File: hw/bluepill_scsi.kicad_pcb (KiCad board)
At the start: 2 copper layers, 43.8 x 73.7 mm, 14 parts, among them J1 Micro_SD_Card, J2 Conn_02x25_Odd_Even, J3 Programming Pins, J4 Berg Power Connector, U1 BluePill_STM32F103C

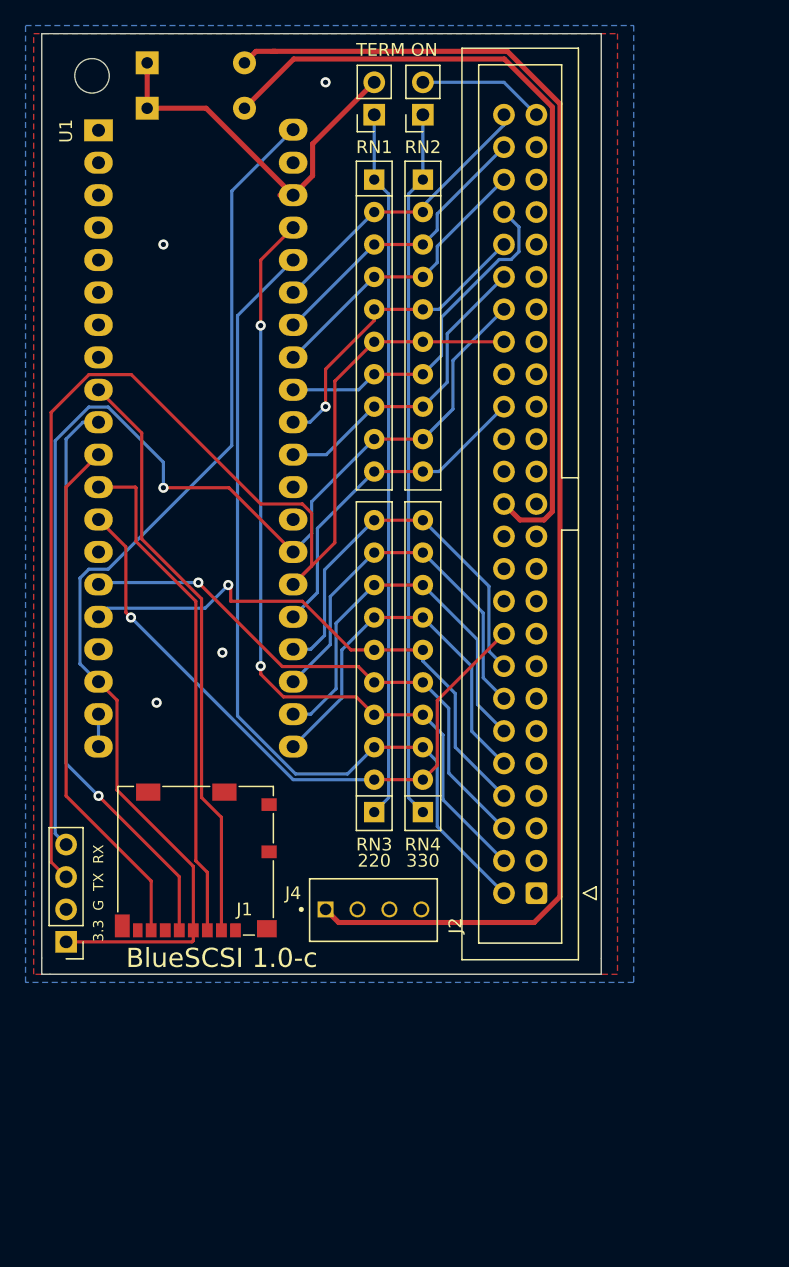
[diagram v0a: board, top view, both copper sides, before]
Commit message: Initial 1.1-a
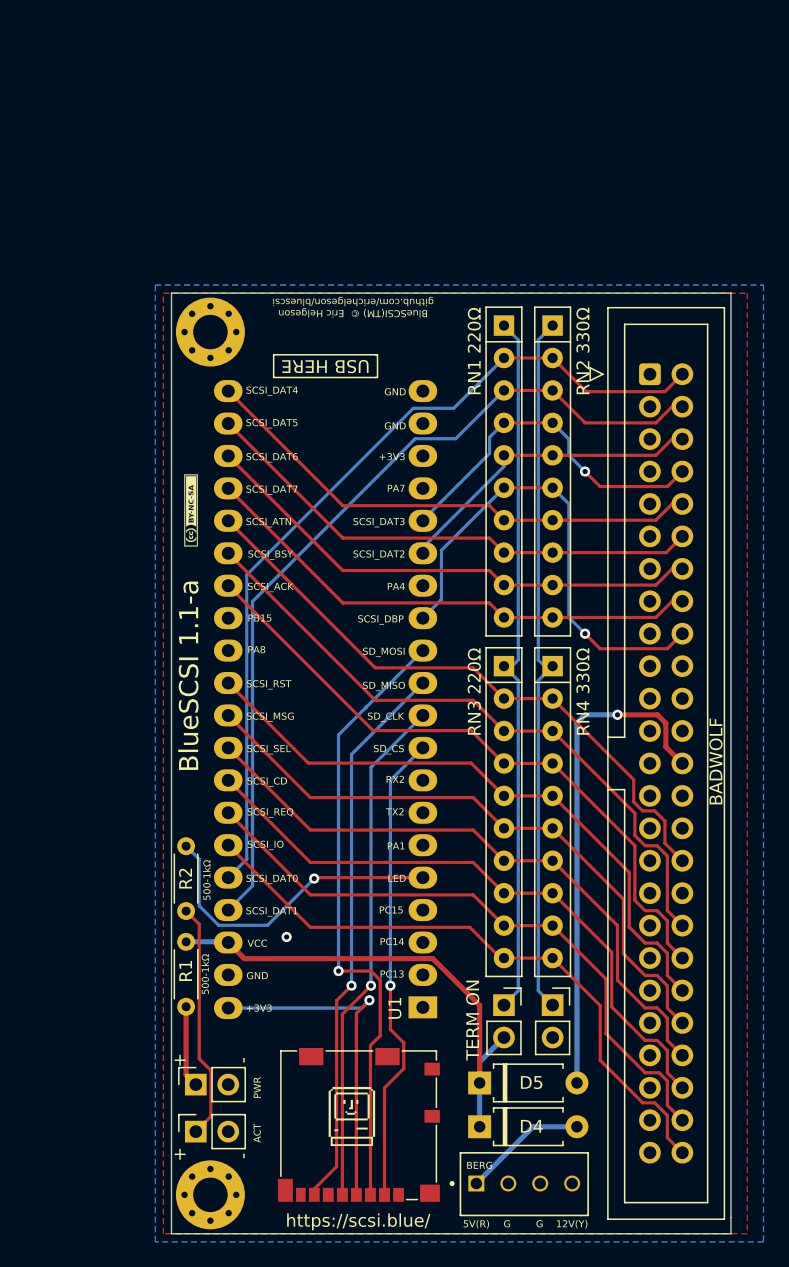
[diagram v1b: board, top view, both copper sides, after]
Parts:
- added G***: LOGO, BlueSCSILogo:dogcow, B.Cu at (95.3, 160.4)
- added G***: LOGO, BlueSCSILogo:mac_happy_small, F.Cu at (95.4, 160.3)
- added G***: LOGO, BlueSCSILogo:cc_by_nc_sa_front_silk_screen, B.Cu at (103.9, 149.4)
- added G***: LOGO, BlueSCSILogo:cc_by_nc_sa_small_front_silk_screen, F.Cu at (82.8, 112.9)
- added G***: LOGO, BlueSCSILogo:BlueSCSILogoFP, B.Cu at (93.2, 126.2)
- added H2: MountingHole_Pad, MountingHole:MountingHole_2.7mm_M2.5_Pad_Via, F.Cu at (84.3, 166.5)
- added J5: Micro_SD_Card, Connector_Card:microSD_HC_Molex_104031-0811, F.Cu at (96.0, 161.0)
- added R1: R_US, Resistor_THT:R_Axial_DIN0204_L3.6mm_D1.6mm_P5.08mm_Horizontal, F.Cu at (82.4, 151.8)
- added R2: R_US, Resistor_THT:R_Axial_DIN0204_L3.6mm_D1.6mm_P5.08mm_Horizontal, F.Cu at (82.4, 144.3)
- D4, D5: moved to F.Cu
- H1: footprint MountingHole:MountingHole_2.7mm_M2.5 -> MountingHole:MountingHole_2.7mm_M2.5_Pad_Via
- J1: value Micro_SD_Card -> Berg Power Connector; footprint Connector_Card:microSD_HC_Molex_104031-0811 -> 171825-4:TE_171825-4
- J3: value Programming Pins -> ACT_LED; footprint Connector_PinHeader_2.54mm:PinHeader_1x04_P2.54mm_Vertical -> Connector_PinSocket_2.54mm:PinSocket_1x02_P2.54mm_Vertical
- J4: value Berg Power Connector -> POWER_LED; footprint 171825-4:TE_171825-4 -> Connector_PinSocket_2.54mm:PinSocket_1x02_P2.54mm_Vertical
- moved D4 87.3 mm to (105.4, 161.2)
- moved D5 80.6 mm to (105.4, 157.7)
- moved U1 73.1 mm to (101.0, 151.8), turned to 180 degrees
- moved JP1 70.5 mm to (111.1, 151.6), turned to 0 degrees
- moved JP2 70.5 mm to (107.3, 151.6), turned to 0 degrees
- moved J2 41.6 mm to (118.7, 102.2), turned to 0 degrees
- moved J1 33.5 mm to (105.2, 165.6), turned to 0 degrees
- moved H1 22.1 mm to (84.3, 98.9)
- moved J3 18.0 mm to (83.2, 161.5), turned to 90 degrees
- moved J4 17.1 mm to (83.2, 157.9), turned to 90 degrees
- moved RN3 15.3 mm to (107.3, 125.1), turned to 270 degrees
- moved RN4 15.3 mm to (111.1, 125.1), turned to 270 degrees
- moved RN1 15.3 mm to (107.3, 98.4)
- moved RN2 15.3 mm to (111.1, 98.4)
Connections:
- J1 pad 1: Net-(J1-Pad1) -> +5V
- J1 pad 2: /SD_CS -> GND
- J1 pad 3: /SD_MOSI -> (no net)
- J1 pad 4: +3V3 -> (no net)
- J2 pad 25: Net-(J2-Pad25) -> (no net)
- J2 pad 34: Net-(J2-Pad34) -> (no net)
- J3 pad 1: +3V3 -> Net-(J3-Pad1)
- J4 pad 1: +5V -> Net-(J4-Pad1)
- RN1 pad 10: /SCSI_ATN -> /SCSI_DAT7
- RN1 pad 2: /SCSI_IO -> /SCSI_DAT0
- RN1 pad 3: /SCSI_REQ -> /SCSI_DAT1
- RN1 pad 4: /SCSI_CD -> /SCSI_DAT3
- RN1 pad 5: /SCSI_MSG -> /SCSI_DAT2
- RN1 pad 6: /SCSI_BSY -> /SCSI_DBP
- RN1 pad 7: /SCSI_SEL -> /SCSI_DAT4
- RN1 pad 8: /SCSI_RST -> /SCSI_DAT5
- RN1 pad 9: /SCSI_ACK -> /SCSI_DAT6
- RN2 pad 10: /SCSI_ATN -> /SCSI_DAT7
- RN2 pad 2: /SCSI_IO -> /SCSI_DAT0
- RN2 pad 3: /SCSI_REQ -> /SCSI_DAT1
- RN2 pad 4: /SCSI_CD -> /SCSI_DAT3
- RN2 pad 5: /SCSI_MSG -> /SCSI_DAT2
- RN2 pad 6: /SCSI_BSY -> /SCSI_DBP
- RN2 pad 7: /SCSI_SEL -> /SCSI_DAT4
- RN2 pad 8: /SCSI_RST -> /SCSI_DAT5
- RN2 pad 9: /SCSI_ACK -> /SCSI_DAT6
- RN3 pad 10: /SCSI_DAT7 -> /SCSI_IO
- RN3 pad 2: /SCSI_DBP -> /SCSI_ATN
- RN3 pad 3: /SCSI_DAT0 -> /SCSI_BSY
- RN3 pad 4: /SCSI_DAT1 -> /SCSI_ACK
- RN3 pad 5: /SCSI_DAT2 -> /SCSI_RST
- RN3 pad 6: /SCSI_DAT3 -> /SCSI_MSG
- RN3 pad 7: /SCSI_DAT4 -> /SCSI_SEL
- RN3 pad 8: /SCSI_DAT5 -> /SCSI_CD
- RN3 pad 9: /SCSI_DAT6 -> /SCSI_REQ
- RN4 pad 10: /SCSI_DAT7 -> /SCSI_IO
- RN4 pad 2: /SCSI_DBP -> /SCSI_ATN
- RN4 pad 3: /SCSI_DAT0 -> /SCSI_BSY
- RN4 pad 4: /SCSI_DAT1 -> /SCSI_ACK
- RN4 pad 5: /SCSI_DAT2 -> /SCSI_RST
- RN4 pad 6: /SCSI_DAT3 -> /SCSI_MSG
- RN4 pad 7: /SCSI_DAT4 -> /SCSI_SEL
- RN4 pad 8: /SCSI_DAT5 -> /SCSI_CD
- RN4 pad 9: /SCSI_DAT6 -> /SCSI_REQ
- U1 pad 1: Net-(U1-Pad1) -> (no net)
- U1 pad 14: Net-(U1-Pad14) -> (no net)
- U1 pad 17: Net-(U1-Pad17) -> (no net)
- U1 pad 2: /LED -> (no net)
- U1 pad 28: Net-(U1-Pad28) -> (no net)
- U1 pad 29: Net-(U1-Pad29) -> (no net)
- U1 pad 3: Net-(U1-Pad3) -> (no net)
- U1 pad 4: Net-(U1-Pad4) -> (no net)
- U1 pad 5: Net-(U1-Pad5) -> /EXTERNAL_LED
- U1 pad 6: Net-(U1-Pad6) -> (no net)
- U1 pad 7: Net-(U1-Pad7) -> (no net)
- U1 pad 8: Net-(U1-Pad8) -> (no net)
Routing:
- net +5V: track 108.7 -> 9.72 mm
- net +3V3: track 85.0 -> 27.0 mm, vias 0 -> 1
- net /SCSI_BSY: track 101.0 -> 51.2 mm
- net /SCSI_ACK: track 85.7 -> 51.2 mm, vias 1 -> 0
- net /SCSI_CD: track 23.0 -> 49.1 mm
- net /SCSI_IO: track 23.0 -> 49.1 mm
- net /SCSI_REQ: track 23.4 -> 49.2 mm
- net /EXTERNAL_LED: track 0.00 -> 24.8 mm, vias 0 -> 1
- net /SCSI_RST: track 24.6 -> 49.1 mm
- net /SCSI_MSG: track 24.6 -> 49.1 mm, vias 1 -> 0
- net /TERM_PWR: track 63.5 -> 39.4 mm, vias 0 -> 1
- net /SCSI_ATN: track 26.3 -> 48.6 mm
- net /SCSI_SEL: track 27.5 -> 49.1 mm
- net Net-(J3-Pad1): track 0.00 -> 18.6 mm
- net /SCSI_DAT2: track 42.8 -> 24.8 mm, vias 1 -> 0
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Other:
- board text added: "+"
- board text added: "+3V3"
- board text added: "-"
- board text added: "12V(Y)"
- board text added: "500-1kΩ"
- board text added: "5V(R)"
- board text added: "ACT"
- board text added: "BADWOLF"
- board text added: "BERG"
- board text added: "BlueSCSI 1.1-a"
- board text added: "BlueSCSI(TM) © Eric Helgeson github.com/erichelgeson/bluescsi"
- board text added: "BlueSCSI(TM) © Eric Helgeson https://github.com/erichelgeson/bluescsi"
- board text added: "G"
- board text added: "GND"
- board text added: "LED"
- board text added: "NOT FOR COMMERCIAL SALE"
- board text added: "PA1"
- board text added: "PA4"
- board text added: "PA7"
- board text added: "PA8"
- board text added: "PB15"
- board text added: "PC13"
- board text added: "PC14"
- board text added: "PC15"
- board text added: "PWR"
- board text added: "RN1 220Ω"
- board text added: "RN2 330Ω"
- board text added: "RN3 220Ω"
- board text added: "RN4 330Ω"
- board text added: "RX2"
- board text added: "SCSI_ACK"
- board text added: "SCSI_ATN"
- board text added: "SCSI_BSY"
- board text added: "SCSI_CD"
- board text added: "SCSI_DAT0"
- board text added: "SCSI_DAT1"
- board text added: "SCSI_DAT2"
- board text added: "SCSI_DAT3"
- board text added: "SCSI_DAT4"
- board text added: "SCSI_DAT5"
- board text added: "SCSI_DAT6"
- board text added: "SCSI_DAT7"
- board text added: "SCSI_DBP"
- board text added: "SCSI_IO"
- board text added: "SCSI_MSG"
- board text added: "SCSI_REQ"
- board text added: "SCSI_RST"
- board text added: "SCSI_SEL"
- board text added: "SD_CLK"
- board text added: "SD_CS"
- board text added: "SD_MISO"
- board text added: "SD_MOSI"
- board text added: "TX2"
- board text added: "USB HERE"
- board text added: "VCC"
- board text added: "https://scsi.blue/"
- board text removed: "220"
- board text removed: "3.3 G TX RX"
- board text removed: "330"
- board text removed: "BlueSCSI 1.0-c"
